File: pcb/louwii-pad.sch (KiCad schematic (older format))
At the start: 38 parts, among them J1 USB_B_Micro, K1 KEYSW, K2 KEYSW, K3 KEYSW, K4 KEYSW, K5 KEYSW, K6 KEYSW, K7 KEYSW, K8 KEYSW, SW1 SW_Push, SW6 Rotary_Encoder_Switch, U1 ATmega32U4-atmel, X1 Crystal

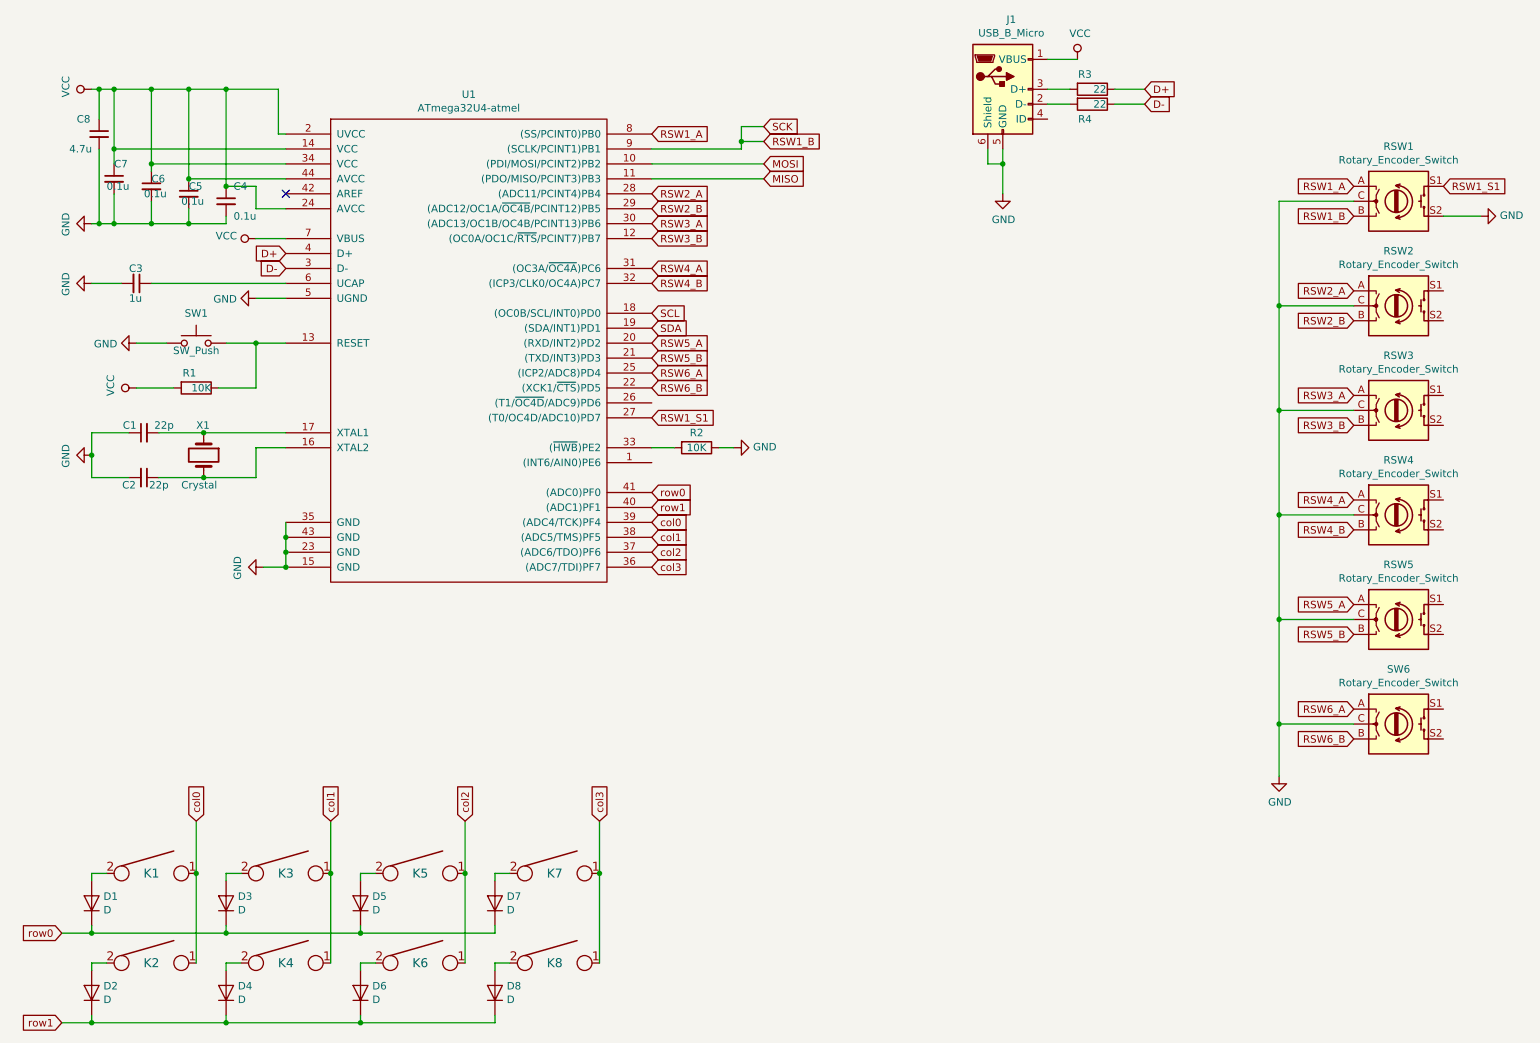
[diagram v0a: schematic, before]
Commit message: add RGB leds - WIP
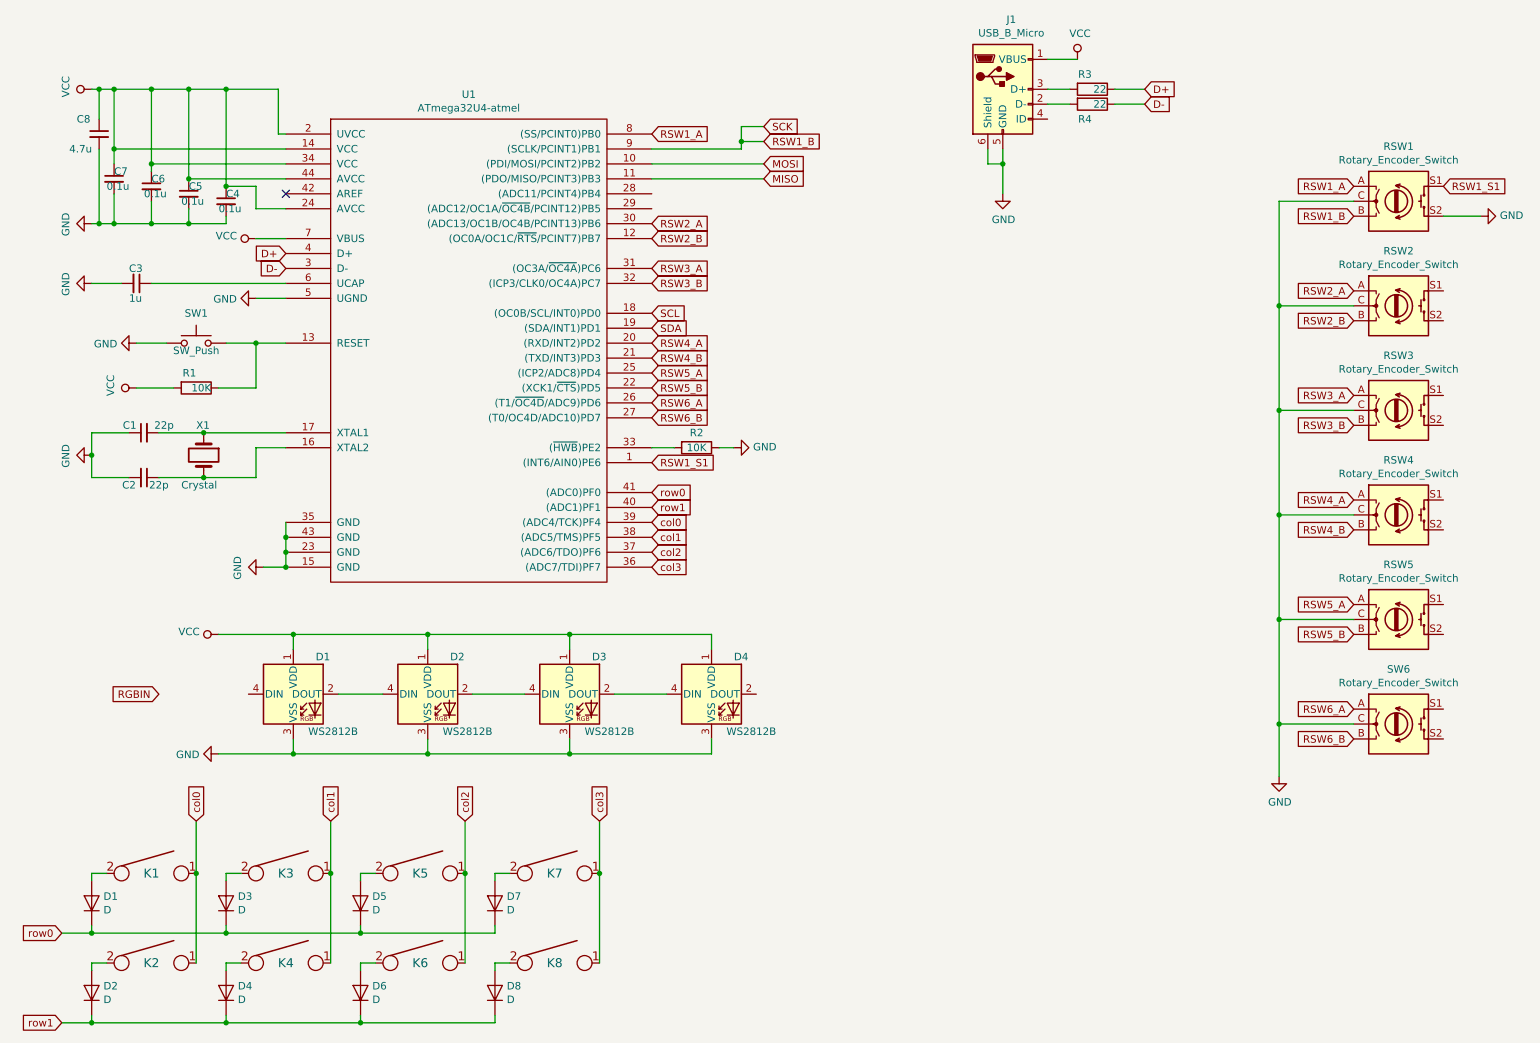
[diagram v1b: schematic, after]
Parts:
- added D1, D2, D3, D4: WS2812B, LED_SMD:LED_WS2812B_PLCC4_5.0x5.0mm_P3.2mm, symbol LED:WS2812B
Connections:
- net GND: now also D1.3 (VSS), D2.3 (VSS), D3.3 (VSS), D4.3 (VSS)
- net RSW1_S1: now also U1.1 ((INT6/AIN0)PE6); no longer U1.27 ((T0/OC4D/ADC10)PD7)
- net RSW2_A: now also U1.30 ((ADC13/OC1B/OC4B/PCINT13)PB6); no longer U1.28 ((ADC11/PCINT4)PB4)
- net RSW2_B: now also U1.12 ((OC0A/OC1C/~RTS~/PCINT7)PB7); no longer U1.29 ((ADC12/OC1A/~OC4B~/PCINT12)PB5)
- net RSW3_A: now also U1.31 ((OC3A/~OC4A~)PC6); no longer U1.30 ((ADC13/OC1B/OC4B/PCINT13)PB6)
- net RSW3_B: now also U1.32 ((ICP3/CLK0/OC4A)PC7); no longer U1.12 ((OC0A/OC1C/~RTS~/PCINT7)PB7)
- net RSW4_A: now also U1.20 ((RXD/INT2)PD2); no longer U1.31 ((OC3A/~OC4A~)PC6)
- net RSW4_B: now also U1.21 ((TXD/INT3)PD3); no longer U1.32 ((ICP3/CLK0/OC4A)PC7)
- net RSW5_A: now also U1.25 ((ICP2/ADC8)PD4); no longer U1.20 ((RXD/INT2)PD2)
- net RSW5_B: now also U1.22 ((XCK1/~CTS~)PD5); no longer U1.21 ((TXD/INT3)PD3)
- net RSW6_A: now also U1.26 ((T1/~OC4D~/ADC9)PD6); no longer U1.25 ((ICP2/ADC8)PD4)
- net RSW6_B: now also U1.27 ((T0/OC4D/ADC10)PD7); no longer U1.22 ((XCK1/~CTS~)PD5)
- net VCC: now also D1.1 (VDD), D2.1 (VDD), D3.1 (VDD), D4.1 (VDD)
- new net: D1.2 (DOUT), D2.4 (DIN)
- new net: D2.2 (DOUT), D3.4 (DIN)
- new net: D3.2 (DOUT), D4.4 (DIN)
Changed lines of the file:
@@
 U 1 1 5DB39D4C
 P 2200 1950
-F 0 "C4" H 2250 2050 50  0000 L CNN
-F 1 "0.1u" H 2250 1850 50  0000 L CNN
+F 0 "C4" H 2200 2000 50  0000 L CNN
+F 1 "0.1u" H 2150 1900 50  0000 L CNN
 F 2 "" H 2200 1950 50  0001 C CNN
 F 3 "~" H 2200 1950 50  0001 C CNN
@@
 U 1 1 5DB3C5CE
 P 1450 1800
-F 0 "C7" H 1450 1900 50  0000 L CNN
+F 0 "C7" H 1450 1850 50  0000 L CNN
 F 1 "0.1u" H 1400 1750 50  0000 L CNN
 F 2 "" H 1450 1800 50  0001 C CNN
@@
 Text GLabel 9750 2050 0    50   Input ~ 0
 RSW1_B
-Text GLabel 5050 1900 2    50   Input ~ 0
+Text GLabel 5050 2100 2    50   Input ~ 0
 RSW2_A
-Text GLabel 5050 2000 2    50   Input ~ 0
+Text GLabel 5050 2200 2    50   Input ~ 0
 RSW2_B
-Text GLabel 5050 2100 2    50   Input ~ 0
+Text GLabel 5050 2400 2    50   Input ~ 0
 RSW3_A
-Text GLabel 5050 2200 2    50   Input ~ 0
+Text GLabel 5050 2500 2    50   Input ~ 0
 RSW3_B
-Text GLabel 5050 2400 2    50   Input ~ 0
+Text GLabel 5050 2900 2    50   Input ~ 0
 RSW4_A
-Text GLabel 5050 2500 2    50   Input ~ 0
+Text GLabel 5050 3000 2    50   Input ~ 0
 RSW4_B
 Connection ~ 9250 4050
@@
 Text GLabel 9750 4850 0    50   Input ~ 0
 RSW5_B
-Text GLabel 5050 2900 2    50   Input ~ 0
+Text GLabel 5050 3100 2    50   Input ~ 0
 RSW5_A
-Text GLabel 5050 3000 2    50   Input ~ 0
+Text GLabel 5050 3200 2    50   Input ~ 0
 RSW5_B
 Wire Wire Line
@@
 Text GLabel 9750 5550 0    50   Input ~ 0
 RSW6_B
-Text GLabel 5050 3100 2    50   Input ~ 0
+Text GLabel 5050 3300 2    50   Input ~ 0
 RSW6_A
-Text GLabel 5050 3200 2    50   Input ~ 0
+Text GLabel 5050 3400 2    50   Input ~ 0
 RSW6_B
 $Comp
@@
 Wire Wire Line
 	10600 2050 10350 2050
-Text GLabel 5050 3400 2    50   Input ~ 0
+Text GLabel 5050 3700 2    50   Input ~ 0
 RSW1_S1
 $Comp
@@
 Wire Wire Line
 	5050 1700 5800 1700
+$Comp
+L LED:WS2812B D1
+U 1 1 5DB4365E
+P 2650 5250
+F 0 "D1" H 2800 5500 50  0000 L CNN
+F 1 "WS2812B" H 2750 5000 50  0000 L CNN
+F 2 "LED_SMD:LED_WS2812B_PLCC4_5.0x5.0mm_P3.2mm" H 2700 4950 50  0001 L TNN
+F 3 "https://cdn-shop.adafruit.com/datasheets/WS2812B.pdf" H 2750 4875 50  0001 L TNN
+	1    2650 5250
+	1    0    0    -1
+$EndComp
+Text GLabel 1750 5250 0    50   Input ~ 0
+RGBIN
+$Comp
+L power:VCC #PWR?
+U 1 1 5DB47967
+P 2150 4850
+F 0 "#PWR?" H 2150 4700 50  0001 C CNN
+F 1 "VCC" V 2168 4977 50  0000 L CNN
+F 2 "" H 2150 4850 50  0001 C CNN
+F 3 "" H 2150 4850 50  0001 C CNN
+	1    2150 4850
+	0    -1   -1   0
+$EndComp
+$Comp
+L power:GND #PWR?
+U 1 1 5DB48DB8
+P 2150 5650
+F 0 "#PWR?" H 2150 5400 50  0001 C CNN
+F 1 "GND" V 2155 5522 50  0000 R CNN
+F 2 "" H 2150 5650 50  0001 C CNN
+F 3 "" H 2150 5650 50  0001 C CNN
+	1    2150 5650
+	0    1    1    0
+$EndComp
+Wire Wire Line
+	2650 4950 2650 4850
+Wire Wire Line
+	2650 4850 2150 4850
+Wire Wire Line
+	2650 5550 2650 5650
+Wire Wire Line
+	2650 5650 2150 5650
+$Comp
+L LED:WS2812B D2
+U 1 1 5DB54C8D
+P 3550 5250
+F 0 "D2" H 3700 5500 50  0000 L CNN
+F 1 "WS2812B" H 3650 5000 50  0000 L CNN
+F 2 "LED_SMD:LED_WS2812B_PLCC4_5.0x5.0mm_P3.2mm" H 3600 4950 50  0001 L TNN
+F 3 "https://cdn-shop.adafruit.com/datasheets/WS2812B.pdf" H 3650 4875 50  0001 L TNN
+	1    3550 5250
+	1    0    0    -1
+$EndComp
+Wire Wire Line
+	3550 4950 3550 4850
+Wire Wire Line
+	3550 4850 2650 4850
+Connection ~ 2650 4850
+Wire Wire Line
+	3550 5550 3550 5650
+Wire Wire Line
+	3550 5650 2650 5650
+Connection ~ 2650 5650
+Wire Wire Line
+	2950 5250 3250 5250
+$Comp
+L LED:WS2812B D3
+U 1 1 5DB6B2F1
+P 4500 5250
+F 0 "D3" H 4650 5500 50  0000 L CNN
+F 1 "WS2812B" H 4600 5000 50  0000 L CNN
+F 2 "LED_SMD:LED_WS2812B_PLCC4_5.0x5.0mm_P3.2mm" H 4550 4950 50  0001 L TNN
+F 3 "https://cdn-shop.adafruit.com/datasheets/WS2812B.pdf" H 4600 4875 50  0001 L TNN
+	1    4500 5250
+	1    0    0    -1
+$EndComp
+Wire Wire Line
+	3850 5250 4200 5250
+Wire Wire Line
+	4500 4950 4500 4850
+Wire Wire Line
+	4500 4850 3550 4850
+Connection ~ 3550 4850
+Wire Wire Line
+	3550 5650 4500 5650
+Wire Wire Line
+	4500 5650 4500 5550
+Connection ~ 3550 5650
+$Comp
+L LED:WS2812B D4
+U 1 1 5DB8349A
+P 5450 5250
+F 0 "D4" H 5600 5500 50  0000 L CNN
+F 1 "WS2812B" H 5550 5000 50  0000 L CNN
+F 2 "LED_SMD:LED_WS2812B_PLCC4_5.0x5.0mm_P3.2mm" H 5500 4950 50  0001 L TNN
+F 3 "https://cdn-shop.adafruit.com/datasheets/WS2812B.pdf" H 5550 4875 50  0001 L TNN
+	1    5450 5250
+	1    0    0    -1
+$EndComp
+Wire Wire Line
+	4500 5650 5450 5650
+Wire Wire Line
+	5450 5650 5450 5550
+Connection ~ 4500 5650
+Wire Wire Line
+	4500 4850 5450 4850
+Wire Wire Line
+	5450 4850 5450 4950
+Connection ~ 4500 4850
+Wire Wire Line
+	4800 5250 5150 5250
 $EndSCHEMATC

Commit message: Finished PCB schematics
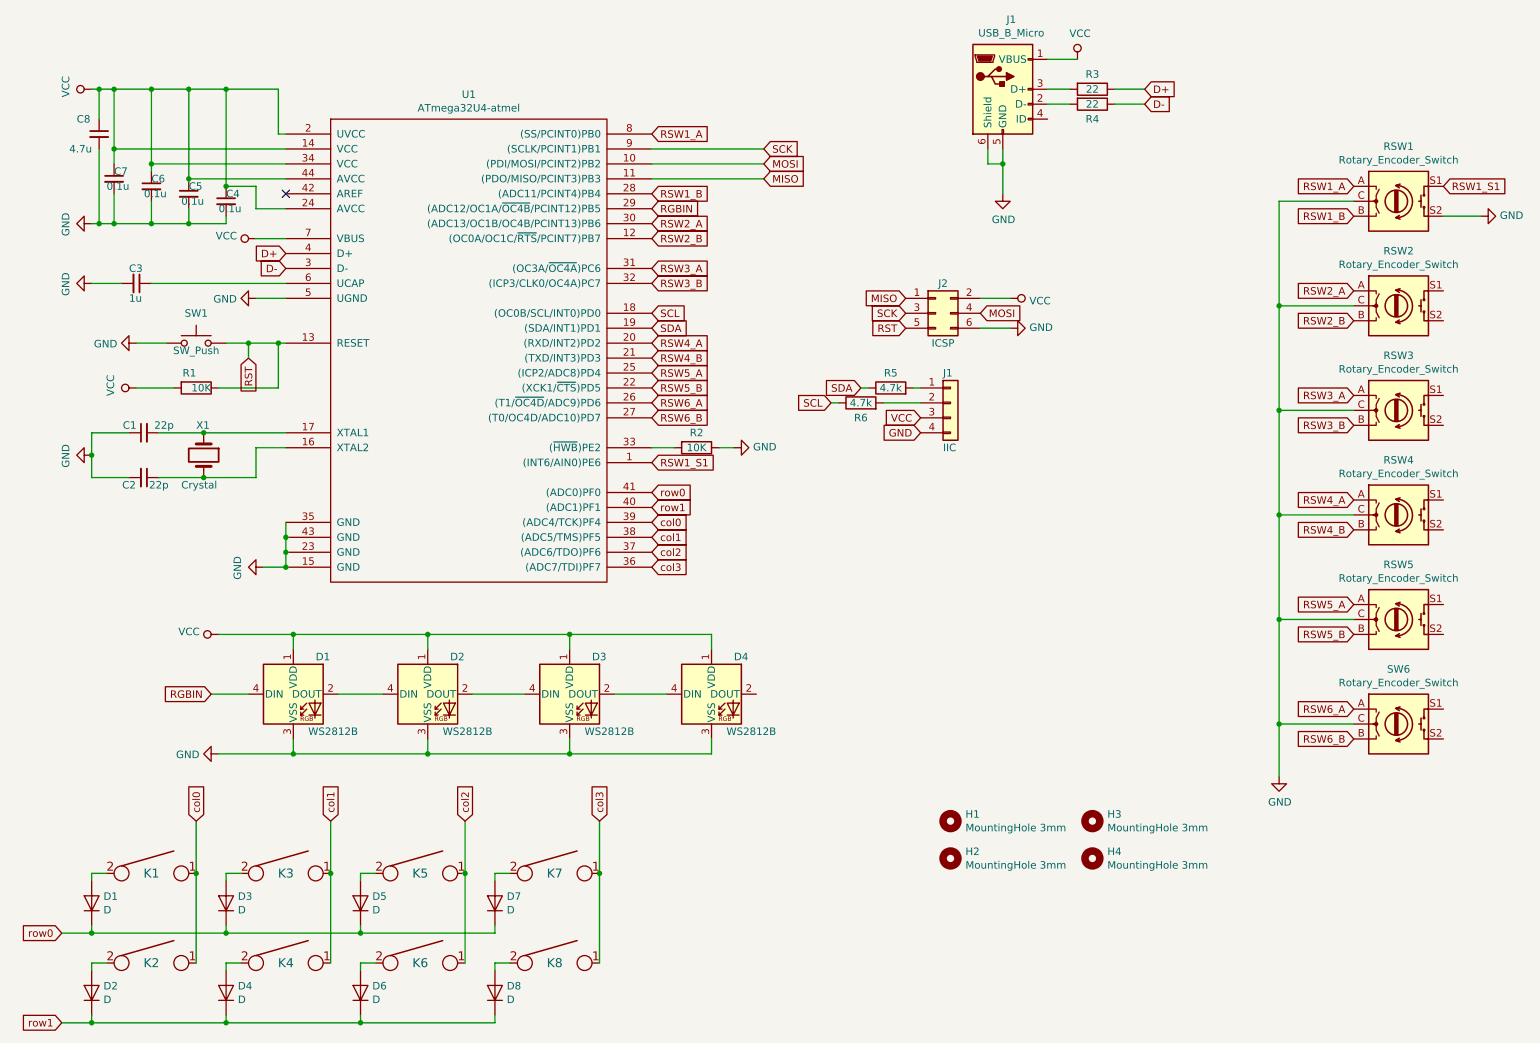
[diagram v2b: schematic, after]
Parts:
- added H1, H2, H3, H4: MountingHole 3mm, symbol Mechanical:MountingHole
- added J1: IIC, symbol Connector_Generic:Conn_01x04
- added J2: ICSP, symbol Connector_Generic:Conn_02x03_Odd_Even
- added R5, R6: 4.7k, symbol Device:R
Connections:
- net GND: now also J1.4 (Pin_4), J2.6 (Pin_6)
- net MISO: now also J2.1 (Pin_1)
- net MOSI: now also J2.4 (Pin_4)
- net RGBIN: now also D1.4 (DIN), U1.29 ((ADC12/OC1A/~OC4B~/PCINT12)PB5)
- net RSW1_B: now also U1.28 ((ADC11/PCINT4)PB4); no longer U1.9 ((SCLK/PCINT1)PB1)
- net SCL: now also R6.1
- net SDA: now also R5.1
- net VCC: now also J1.3 (Pin_3), J2.2 (Pin_2)
- net RST: now reaches R1.1, SW1.2, U1.13 (RESET)
- net RST: now also J2.5 (Pin_5)
- new net: J1.1 (Pin_1), R5.2
- new net: J1.2 (Pin_2), R6.2
- new net SCK: J2.3 (Pin_3), U1.9 ((SCLK/PCINT1)PB1)
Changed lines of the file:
@@
 U 1 1 5DB19524
 P 8000 1200
-F 0 "R3" V 7900 1150 50  0000 C CNN
-F 1 "22" V 8000 1250 50  0000 C CNN
+F 0 "R3" V 7900 1200 50  0000 C CNN
+F 1 "22" V 8000 1200 50  0000 C CNN
 F 2 "" V 7930 1200 50  0001 C CNN
 F 3 "~" H 8000 1200 50  0001 C CNN
@@
 U 1 1 5DB1C383
 P 8000 1300
-F 0 "R4" V 8100 1250 50  0000 C CNN
-F 1 "22" V 8000 1350 50  0000 C CNN
+F 0 "R4" V 8100 1300 50  0000 C CNN
+F 1 "22" V 8000 1300 50  0000 C CNN
 F 2 "" V 7930 1300 50  0001 C CNN
 F 3 "~" H 8000 1300 50  0001 C CNN
@@
 Text GLabel 5050 1500 2    50   Input ~ 0
 RSW1_A
-Text GLabel 5800 1550 2    50   Input ~ 0
+Text GLabel 5050 1900 2    50   Input ~ 0
 RSW1_B
 Text GLabel 9750 1850 0    50   Input ~ 0
@@
 	1850 3200 1600 3200
 Wire Wire Line
-	2200 2900 2400 2900
-Wire Wire Line
-	2400 2900 2400 3200
-Wire Wire Line
-	2400 3200 2150 3200
-Connection ~ 2400 2900
-Wire Wire Line
-	2400 2900 2600 2900
-Wire Wire Line
 	2600 2500 1700 2500
 Wire Wire Line
@@
 Wire Wire Line
 	2200 1200 2550 1200
-Wire Wire Line
-	5050 1600 5650 1600
-Wire Wire Line
-	5650 1600 5650 1550
-Wire Wire Line
-	5650 1550 5800 1550
 Text GLabel 5800 1800 2    50   Input ~ 0
 MISO
-Text GLabel 5800 1450 2    50   Input ~ 0
+Text GLabel 5800 1600 2    50   Input ~ 0
 SCK
 Text GLabel 5800 1700 2    50   Input ~ 0
 MOSI
-Wire Wire Line
-	5800 1450 5650 1450
-Wire Wire Line
-	5650 1450 5650 1550
-Connection ~ 5650 1550
 Wire Wire Line
 	5050 1800 5800 1800
@@
 	1    0    0    -1
 $EndComp
-Text GLabel 1750 5250 0    50   Input ~ 0
+Text GLabel 2100 5250 0    50   Input ~ 0
 RGBIN
 $Comp
@@
 Wire Wire Line
 	4800 5250 5150 5250
+Text GLabel 5050 2000 2    50   Input ~ 0
+RGBIN
+$Comp
+L Connector_Generic:Conn_02x03_Odd_Even J2
+U 1 1 5DB2C169
+P 6950 2700
+F 0 "J2" H 7000 2900 50  0000 C CNN
+F 1 "ICSP" H 7000 2500 50  0000 C CNN
+F 2 "" H 6950 2700 50  0001 C CNN
+F 3 "~" H 6950 2700 50  0001 C CNN
+	1    6950 2700
+	1    0    0    -1
+$EndComp
+$Comp
+L Connector_Generic:Conn_01x04 J1
+U 1 1 5DB2DC0B
+P 7050 3300
+F 0 "J1" H 7000 3500 50  0000 L CNN
+F 1 "IIC" H 7000 3000 50  0000 L CNN
+F 2 "" H 7050 3300 50  0001 C CNN
+F 3 "~" H 7050 3300 50  0001 C CNN
+	1    7050 3300
+	1    0    0    -1
+$EndComp
+Text GLabel 6450 3200 0    50   Input ~ 0
+SDA
+Text GLabel 6250 3300 0    50   Input ~ 0
+SCL
+Text GLabel 6850 3400 0    50   Input ~ 0
+VCC
+Text GLabel 6850 3500 0    50   Input ~ 0
+GND
+Wire Wire Line
+	5800 1600 5050 1600
+Text GLabel 6750 2600 0    50   Input ~ 0
+MISO
+Text GLabel 6750 2700 0    50   Input ~ 0
+SCK
+Text GLabel 2350 3000 3    50   Input ~ 0
+RST
+Text GLabel 6750 2800 0    50   Input ~ 0
+RST
+$Comp
+L power:VCC #PWR?
+U 1 1 5DB56B8F
+P 7450 2600
+F 0 "#PWR?" H 7450 2450 50  0001 C CNN
+F 1 "VCC" V 7467 2728 50  0000 L CNN
+F 2 "" H 7450 2600 50  0001 C CNN
+F 3 "" H 7450 2600 50  0001 C CNN
+	1    7450 2600
+	0    1    1    0
+$EndComp
+Wire Wire Line
+	7250 2600 7450 2600
+Text GLabel 7250 2700 2    50   Input ~ 0
+MOSI
+$Comp
+L power:GND #PWR?
+U 1 1 5DB5E936
+P 7450 2800
+F 0 "#PWR?" H 7450 2550 50  0001 C CNN
+F 1 "GND" V 7455 2672 50  0000 R CNN
+F 2 "" H 7450 2800 50  0001 C CNN
+F 3 "" H 7450 2800 50  0001 C CNN
+	1    7450 2800
+	0    -1   -1   0
+$EndComp
+Wire Wire Line
+	7450 2800 7250 2800
+Wire Wire Line
+	2200 2900 2350 2900
+Wire Wire Line
+	2550 2900 2550 3200
+Wire Wire Line
+	2550 3200 2150 3200
+Connection ~ 2550 2900
+Wire Wire Line
+	2550 2900 2600 2900
+Wire Wire Line
+	2350 3000 2350 2900
+Connection ~ 2350 2900
+Wire Wire Line
+	2350 2900 2550 2900
+$Comp
+L Device:R R5
+U 1 1 5DBA043E
+P 6650 3200
+F 0 "R5" V 6750 3200 50  0000 C CNN
+F 1 "4.7k" V 6650 3200 50  0000 C CNN
+F 2 "" V 6580 3200 50  0001 C CNN
+F 3 "~" H 6650 3200 50  0001 C CNN
+	1    6650 3200
+	0    -1   -1   0
+$EndComp
+Wire Wire Line
+	6850 3200 6800 3200
+Wire Wire Line
+	6500 3200 6450 3200
+$Comp
+L Device:R R6
+U 1 1 5DBB4BB8
+P 6450 3300
+F 0 "R6" V 6350 3300 50  0000 C CNN
+F 1 "4.7k" V 6450 3300 50  0000 C CNN
+F 2 "" V 6380 3300 50  0001 C CNN
+F 3 "~" H 6450 3300 50  0001 C CNN
+	1    6450 3300
+	0    -1   -1   0
+$EndComp
+Wire Wire Line
+	6850 3300 6600 3300
+Wire Wire Line
+	6300 3300 6250 3300
+$Comp
+L Mechanical:MountingHole H2
+U 1 1 5DBCEBB2
+P 7050 6350
+F 0 "H2" H 7150 6396 50  0000 L CNN
+F 1 "MountingHole 3mm" H 7150 6305 50  0000 L CNN
+F 2 "" H 7050 6350 50  0001 C CNN
+F 3 "~" H 7050 6350 50  0001 C CNN
+	1    7050 6350
+	1    0    0    -1
+$EndComp
+$Comp
+L Mechanical:MountingHole H1
+U 1 1 5DBD03B9
+P 7050 6100
+F 0 "H1" H 7150 6146 50  0000 L CNN
+F 1 "MountingHole 3mm" H 7150 6055 50  0000 L CNN
+F 2 "" H 7050 6100 50  0001 C CNN
+F 3 "~" H 7050 6100 50  0001 C CNN
+	1    7050 6100
+	1    0    0    -1
+$EndComp
+$Comp
+L Mechanical:MountingHole H3
+U 1 1 5DBD705C
+P 8000 6100
+F 0 "H3" H 8100 6146 50  0000 L CNN
+F 1 "MountingHole 3mm" H 8100 6055 50  0000 L CNN
+F 2 "" H 8000 6100 50  0001 C CNN
+F 3 "~" H 8000 6100 50  0001 C CNN
+	1    8000 6100
+	1    0    0    -1
+$EndComp
+$Comp
+L Mechanical:MountingHole H4
+U 1 1 5DBDD73C
+P 8000 6350
+F 0 "H4" H 8100 6396 50  0000 L CNN
+F 1 "MountingHole 3mm" H 8100 6305 50  0000 L CNN
+F 2 "" H 8000 6350 50  0001 C CNN
+F 3 "~" H 8000 6350 50  0001 C CNN
+	1    8000 6350
+	1    0    0    -1
+$EndComp
+Wire Wire Line
+	2350 5250 2100 5250
 $EndSCHEMATC
